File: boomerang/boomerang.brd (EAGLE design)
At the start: 34.3 x 31.8 mm, 11 parts, among them IC1 WS2811-SOP8

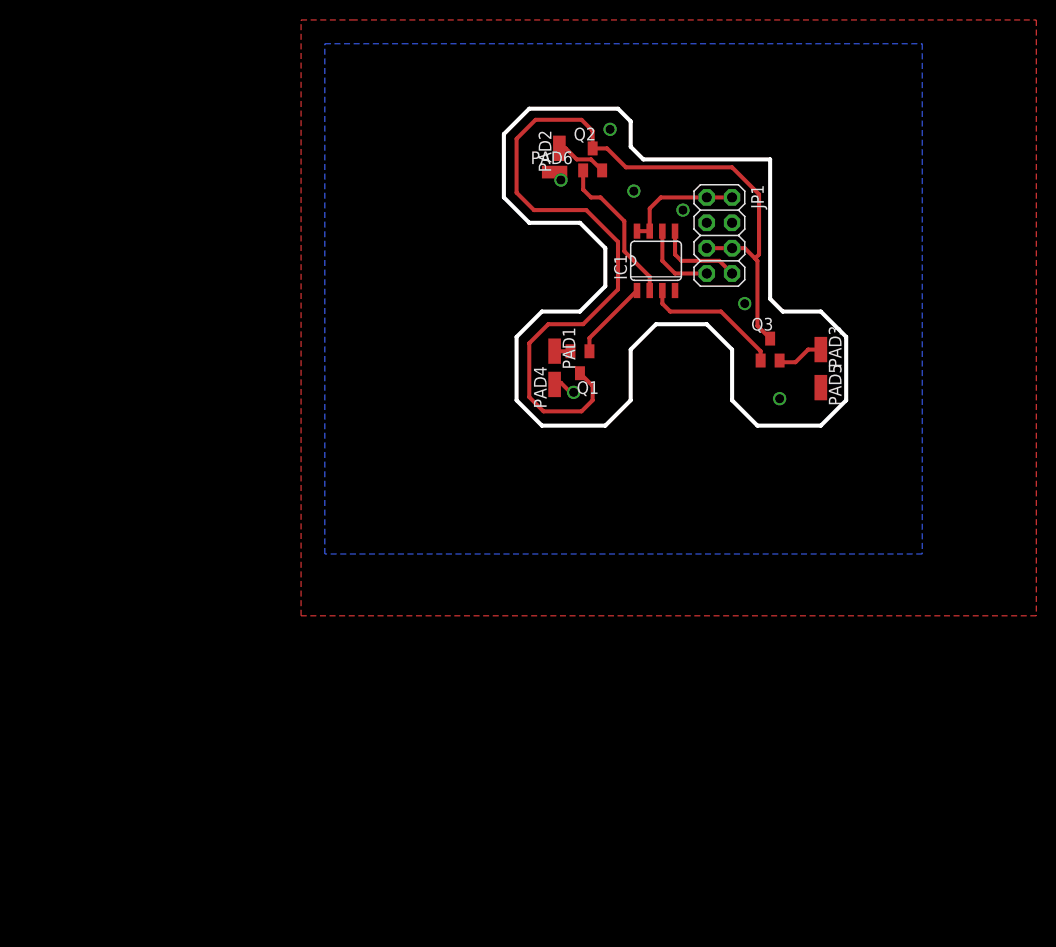
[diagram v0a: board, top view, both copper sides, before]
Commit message: nicer :)
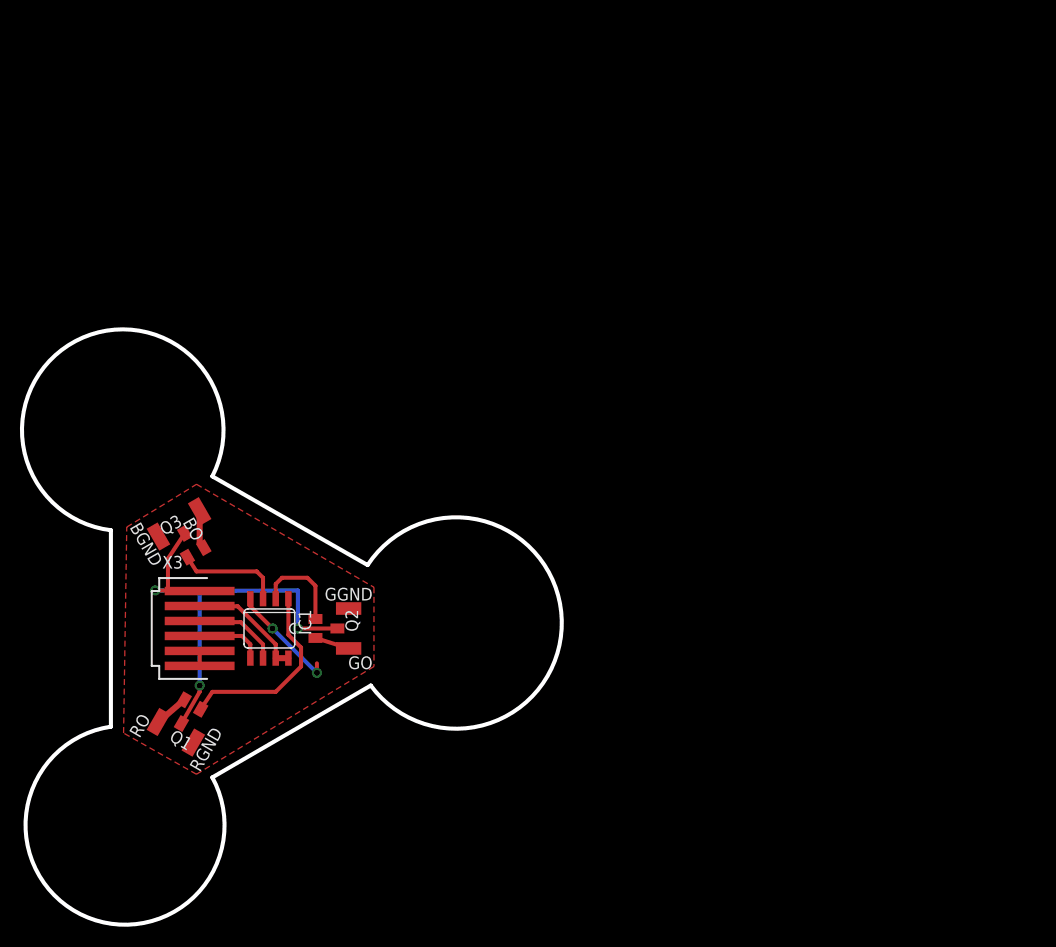
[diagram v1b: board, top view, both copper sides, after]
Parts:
- removed JP1: (no value), adafruit:2X04
- removed PAD1, PAD2, PAD3, PAD4, PAD5, PAD6: (no value), wirepad:SMD1,27-2,54
- added BGND, BO, GGND, GO, RGND, RO: (no value), wirepad:SMD1,27-2,54
- added X3: 87438-06, con-molex:87438-06
- moved Q3 61.2 mm to (-4.76, 8.57), turned to 30 degrees
- moved Q2 54.0 mm to (8.89, 0.00), turned to 270 degrees
- moved IC1 53.4 mm to (3.17, 0.00), turned to 180 degrees
- moved Q1 52.8 mm to (-5.08, -8.57), turned to 150 degrees
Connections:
- net N$1 renamed R
- net N$2 renamed G
- net N$3 renamed B
- removed net N$10: IC1.5, JP1.8
- removed net N$5: IC1.6, JP1.7
- removed net N$6: PAD2.1, Q2.2
- removed net N$7: PAD1.1, Q1.2
- removed net N$9: PAD3.1, Q3.2
- new net BO: BO.1, Q3.2
- new net DIN: IC1.6, X3.3
- new net DO: IC1.5, X3.4
- new net GO: GO.1, Q2.2
- new net RO: Q1.2, RO.1
- net 3V3: now also X3.1; no longer JP1.5, JP1.6
- net GND: now also BGND.1, GGND.1, RGND.1, X3.5, X3.6; no longer JP1.3, JP1.4, PAD4.1, PAD5.1, PAD6.1
- net VCC: now also X3.2; no longer JP1.1, JP1.2
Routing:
- net 3V3: track 99.2 -> 49.7 mm, vias 0 -> 3
- net R: track 8.06 -> 19.4 mm
- net GND: track 2.68 -> 12.6 mm, vias 7 -> 2
- net N$10: track 8.84 -> 0.00 mm
- net DIN: track 0.00 -> 8.70 mm
- net N$5: track 7.94 -> 0.00 mm
- net DO: track 0.00 -> 6.81 mm
- net G: track 15.4 -> 9.37 mm
- net N$6: track 5.20 -> 0.00 mm
- net N$9: track 4.73 -> 0.00 mm
- net BO: track 0.00 -> 3.83 mm
- net GO: track 0.00 -> 3.49 mm
- net RO: track 0.00 -> 3.41 mm
- net B: track 14.1 -> 10.7 mm
- net N$7: track 1.59 -> 0.00 mm
- removed copper zone on layer 16, net GND
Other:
- board size 34.3 x 31.8 mm -> 54.1 x 59.6 mm
